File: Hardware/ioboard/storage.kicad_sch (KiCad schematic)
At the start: 8 parts, among them U4 W25Q32JV

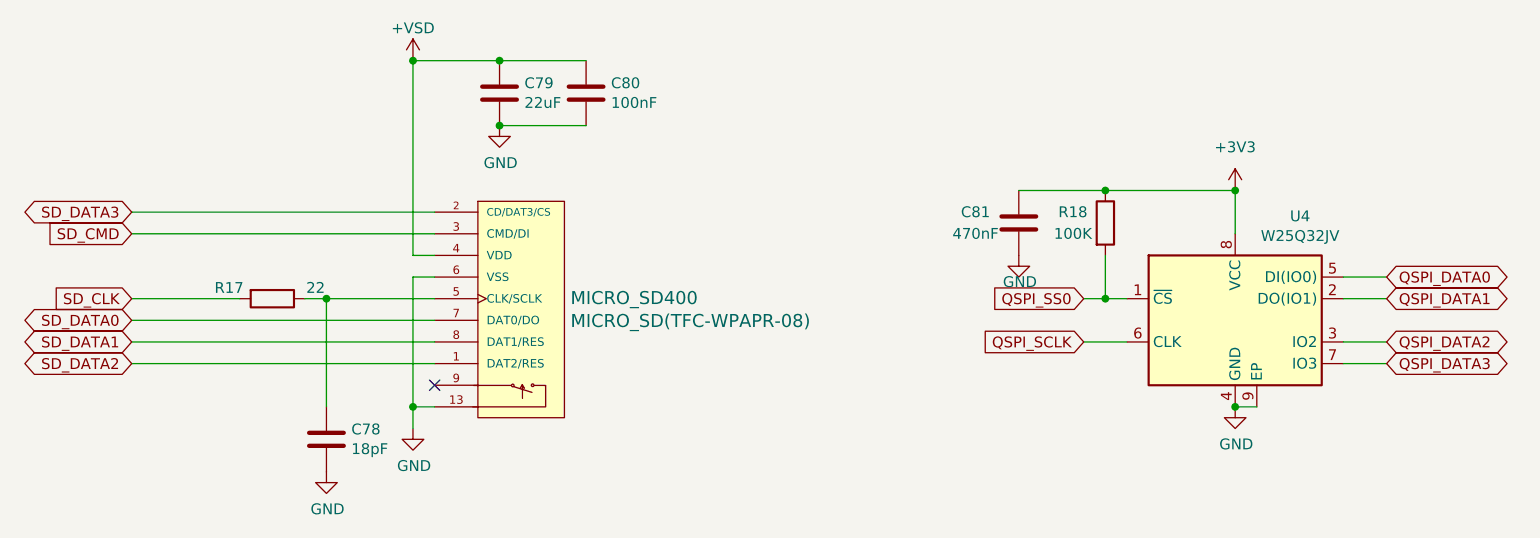
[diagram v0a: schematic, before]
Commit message: Design grip flex, SB/IOB WIP
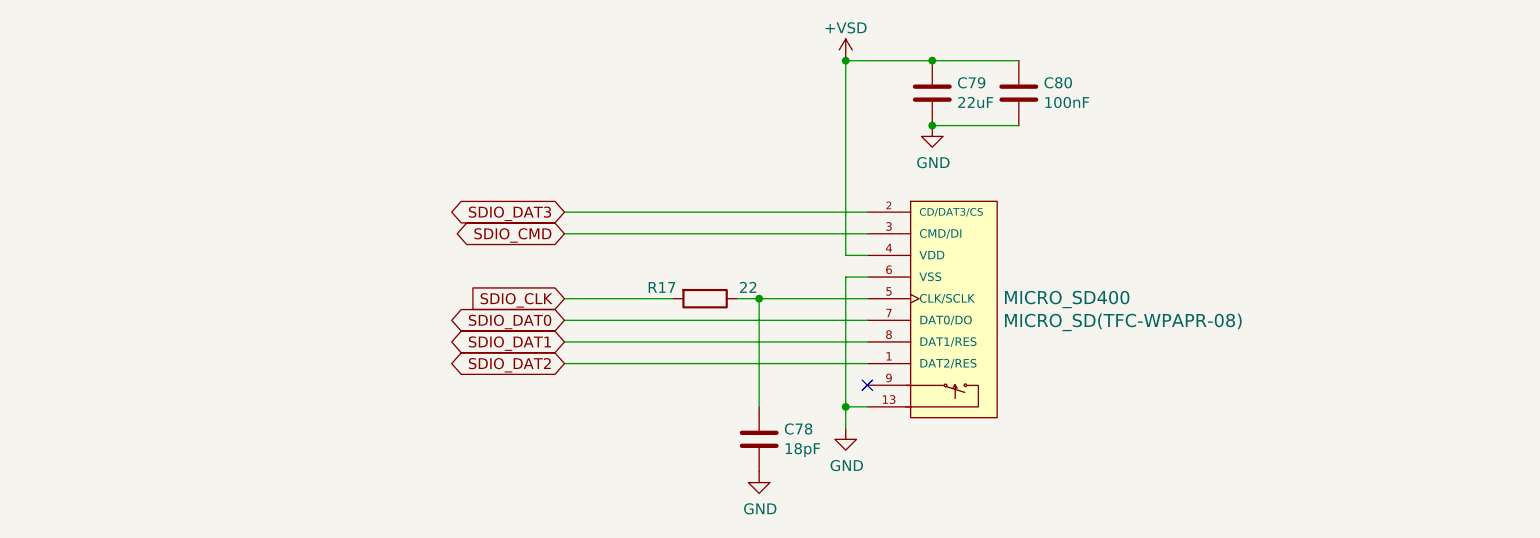
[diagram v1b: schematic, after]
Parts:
- removed C81: 470nF, Capacitor_SMD:C_0402_1005Metric, symbol Device:C
- removed R18: 100K, Resistor_SMD:R_0402_1005Metric, symbol Device:R
- removed U4: W25Q32JV, Package_SON:WSON-8-1EP_6x5mm_P1.27mm_EP3.4x4.3mm, symbol Memory_Flash:W25Q32JVZP
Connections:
- net SD_CLK renamed SDIO_CLK
- net SD_CMD renamed SDIO_CMD
- net SD_DATA0 renamed SDIO_DAT0
- net SD_DATA1 renamed SDIO_DAT1
- net SD_DATA2 renamed SDIO_DAT2
- net SD_DATA3 renamed SDIO_DAT3
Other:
- moved on the sheet: C78, C79, C80, MICRO_SD400, R17
